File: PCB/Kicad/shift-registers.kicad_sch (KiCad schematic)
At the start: 6 parts

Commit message: Arduino mega retrofit WIP
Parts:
- U-LEDS1, UVU-LINE1, UVU-LINE2, UVU-LINE3, UVU-MASTER-L1, UVU-MASTER-R1: footprint Package_DIP:DIP-16_W7.62mm_LongPads -> Package_SO:SO-16_3.9x9.9mm_P1.27mm
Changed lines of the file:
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@@
     (property "Reference" "UVU-LINE1" (id 0) (at 41.91 72.39 0))
     (property "Value" "74HC595" (id 1) (at 40.64 102.87 0))
-    (property "Footprint" "Package_DIP:DIP-16_W7.62mm_LongPads" (id 2) (at 41.91 95.25 0)
+    (property "Footprint" "Package_SO:SO-16_3.9x9.9mm_P1.27mm" (id 2) (at 41.91 95.25 0)
       (effects (font (size 1.27 1.27)) hide)
     )
@@
     (property "Reference" "UVU-LINE2" (id 0) (at 81.28 72.644 0))
     (property "Value" "74HC595" (id 1) (at 80.01 103.124 0))
-    (property "Footprint" "Package_DIP:DIP-16_W7.62mm_LongPads" (id 2) (at 81.28 95.25 0)
+    (property "Footprint" "Package_SO:SO-16_3.9x9.9mm_P1.27mm" (id 2) (at 81.28 95.25 0)
       (effects (font (size 1.27 1.27)) hide)
     )
@@
     (property "Reference" "UVU-LINE3" (id 0) (at 123.19 72.39 0))
     (property "Value" "74HC595" (id 1) (at 121.92 102.87 0))
-    (property "Footprint" "Package_DIP:DIP-16_W7.62mm_LongPads" (id 2) (at 123.19 95.25 0)
+    (property "Footprint" "Package_SO:SO-16_3.9x9.9mm_P1.27mm" (id 2) (at 123.19 95.25 0)
       (effects (font (size 1.27 1.27)) hide)
     )
@@
     (property "Reference" "UVU-MASTER-L1" (id 0) (at 161.29 72.39 0))
     (property "Value" "74HC595" (id 1) (at 160.02 102.87 0))
-    (property "Footprint" "Package_DIP:DIP-16_W7.62mm_LongPads" (id 2) (at 161.29 95.25 0)
+    (property "Footprint" "Package_SO:SO-16_3.9x9.9mm_P1.27mm" (id 2) (at 161.29 95.25 0)
       (effects (font (size 1.27 1.27)) hide)
     )
@@
     (property "Reference" "UVU-MASTER-R1" (id 0) (at 200.66 72.39 0))
     (property "Value" "74HC595" (id 1) (at 199.39 102.87 0))
-    (property "Footprint" "Package_DIP:DIP-16_W7.62mm_LongPads" (id 2) (at 200.66 95.25 0)
+    (property "Footprint" "Package_SO:SO-16_3.9x9.9mm_P1.27mm" (id 2) (at 200.66 95.25 0)
       (effects (font (size 1.27 1.27)) hide)
     )
@@
     (property "Reference" "U-LEDS1" (id 0) (at 247.65 72.39 0))
     (property "Value" "74HC595" (id 1) (at 246.38 102.87 0))
-    (property "Footprint" "Package_DIP:DIP-16_W7.62mm_LongPads" (id 2) (at 247.65 95.25 0)
+    (property "Footprint" "Package_SO:SO-16_3.9x9.9mm_P1.27mm" (id 2) (at 247.65 95.25 0)
       (effects (font (size 1.27 1.27)) hide)
     )

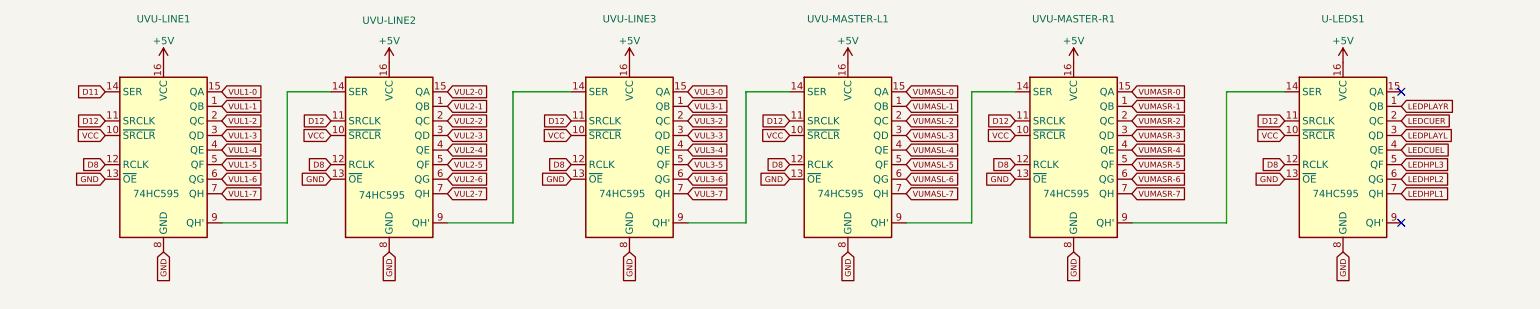
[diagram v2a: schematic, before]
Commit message: trillbar added
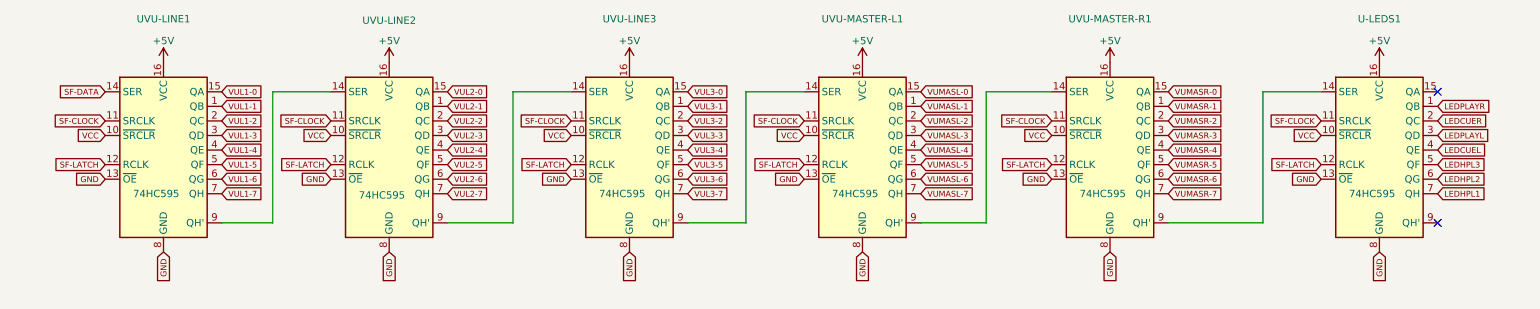
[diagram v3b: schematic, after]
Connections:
- net D11 renamed SF-DATA
- net D12 renamed SF-CLOCK
- net D8 renamed SF-LATCH
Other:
- moved on the sheet: U-LEDS1, UVU-MASTER-L1, UVU-MASTER-R1

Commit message: board updated
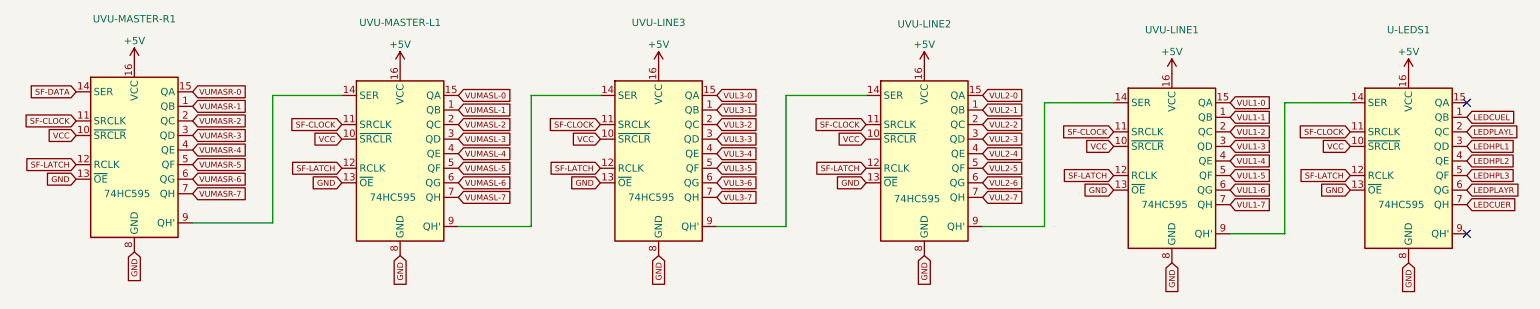
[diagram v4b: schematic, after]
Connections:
- net LEDCUEL: now also U-LEDS1.1 (QB); no longer U-LEDS1.4 (QE)
- net LEDCUER: now also U-LEDS1.7 (QH); no longer U-LEDS1.2 (QC)
- net LEDHPL1: now also U-LEDS1.3 (QD); no longer U-LEDS1.7 (QH)
- net LEDHPL2: now also U-LEDS1.4 (QE); no longer U-LEDS1.6 (QG)
- net LEDPLAYL: now also U-LEDS1.2 (QC); no longer U-LEDS1.3 (QD)
- net LEDPLAYR: now also U-LEDS1.6 (QG); no longer U-LEDS1.1 (QB)
- net SF-DATA: now also UVU-MASTER-R1.14 (SER); no longer UVU-LINE1.14 (SER)
- net at UVU-LINE1.9 (QH'): now also U-LEDS1.14 (SER); no longer UVU-LINE2.14 (SER)
- net at UVU-LINE2.9 (QH'): now also UVU-LINE1.14 (SER); no longer UVU-LINE3.14 (SER)
- net at UVU-LINE3.9 (QH'): now also UVU-LINE2.14 (SER); no longer UVU-MASTER-L1.14 (SER)
- net at UVU-MASTER-L1.9 (QH'): now also UVU-LINE3.14 (SER); no longer UVU-MASTER-R1.14 (SER)
- net at UVU-MASTER-R1.9 (QH'): now also UVU-MASTER-L1.14 (SER); no longer U-LEDS1.14 (SER)
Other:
- moved on the sheet: U-LEDS1, UVU-LINE1, UVU-LINE2, UVU-LINE3, UVU-MASTER-L1, UVU-MASTER-R1

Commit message: fixing 3dmodels
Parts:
- U-LEDS1, UVU-LINE1, UVU-LINE2, UVU-LINE3, UVU-MASTER-L1, UVU-MASTER-R1: footprint Package_SO:SO-16_3.9x9.9mm_P1.27mm -> Library:SO-16_3.9x9.9mm_P1.27mm
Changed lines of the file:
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@@
     (property "Reference" "UVU-MASTER-R1" (id 0) (at 36.83 72.39 0))
     (property "Value" "74HC595" (id 1) (at 35.56 102.87 0))
-    (property "Footprint" "Package_SO:SO-16_3.9x9.9mm_P1.27mm" (id 2) (at 36.83 95.25 0)
+    (property "Footprint" "Library:SO-16_3.9x9.9mm_P1.27mm" (id 2) (at 36.83 95.25 0)
       (effects (font (size 1.27 1.27)) hide)
     )
@@
     (property "Reference" "UVU-MASTER-L1" (id 0) (at 83.185 73.025 0))
     (property "Value" "74HC595" (id 1) (at 81.915 103.505 0))
-    (property "Footprint" "Package_SO:SO-16_3.9x9.9mm_P1.27mm" (id 2) (at 83.185 95.885 0)
+    (property "Footprint" "Library:SO-16_3.9x9.9mm_P1.27mm" (id 2) (at 83.185 95.885 0)
       (effects (font (size 1.27 1.27)) hide)
     )
@@
     (property "Reference" "UVU-LINE3" (id 0) (at 128.27 73.025 0))
     (property "Value" "74HC595" (id 1) (at 127 103.505 0))
-    (property "Footprint" "Package_SO:SO-16_3.9x9.9mm_P1.27mm" (id 2) (at 128.27 95.885 0)
+    (property "Footprint" "Library:SO-16_3.9x9.9mm_P1.27mm" (id 2) (at 128.27 95.885 0)
       (effects (font (size 1.27 1.27)) hide)
     )
@@
     (property "Reference" "UVU-LINE2" (id 0) (at 174.625 73.279 0))
     (property "Value" "74HC595" (id 1) (at 173.355 103.759 0))
-    (property "Footprint" "Package_SO:SO-16_3.9x9.9mm_P1.27mm" (id 2) (at 174.625 95.885 0)
+    (property "Footprint" "Library:SO-16_3.9x9.9mm_P1.27mm" (id 2) (at 174.625 95.885 0)
       (effects (font (size 1.27 1.27)) hide)
     )
@@
     (property "Reference" "UVU-LINE1" (id 0) (at 217.805 74.295 0))
     (property "Value" "74HC595" (id 1) (at 216.535 104.775 0))
-    (property "Footprint" "Package_SO:SO-16_3.9x9.9mm_P1.27mm" (id 2) (at 217.805 97.155 0)
+    (property "Footprint" "Library:SO-16_3.9x9.9mm_P1.27mm" (id 2) (at 217.805 97.155 0)
       (effects (font (size 1.27 1.27)) hide)
     )
@@
     (property "Reference" "U-LEDS1" (id 0) (at 259.08 74.295 0))
     (property "Value" "74HC595" (id 1) (at 257.81 104.775 0))
-    (property "Footprint" "Package_SO:SO-16_3.9x9.9mm_P1.27mm" (id 2) (at 259.08 97.155 0)
+    (property "Footprint" "Library:SO-16_3.9x9.9mm_P1.27mm" (id 2) (at 259.08 97.155 0)
       (effects (font (size 1.27 1.27)) hide)
     )
